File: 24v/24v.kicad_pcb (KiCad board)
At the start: 2 copper layers, 82.6 x 50.8 mm, 51 parts, among them J1 Conn_01x08_Female, J2 Conn_01x01, J3 Conn_02x08_Counter_Clockwise, J4 Conn_02x08_Counter_Clockwise, J5 Conn_01x01, J6 Conn_02x08_Counter_Clockwise, J7 Conn_02x08_Counter_Clockwise, Q1 FET_A_UP, Q2 FET_A_DOWN, Q3 FET_B_UP, Q4 FET_B_DOWN, U1 7400, U2 IRS2108, U3 TLP2955, U4 TLP2955, U5 IRS2108, U6 L7812

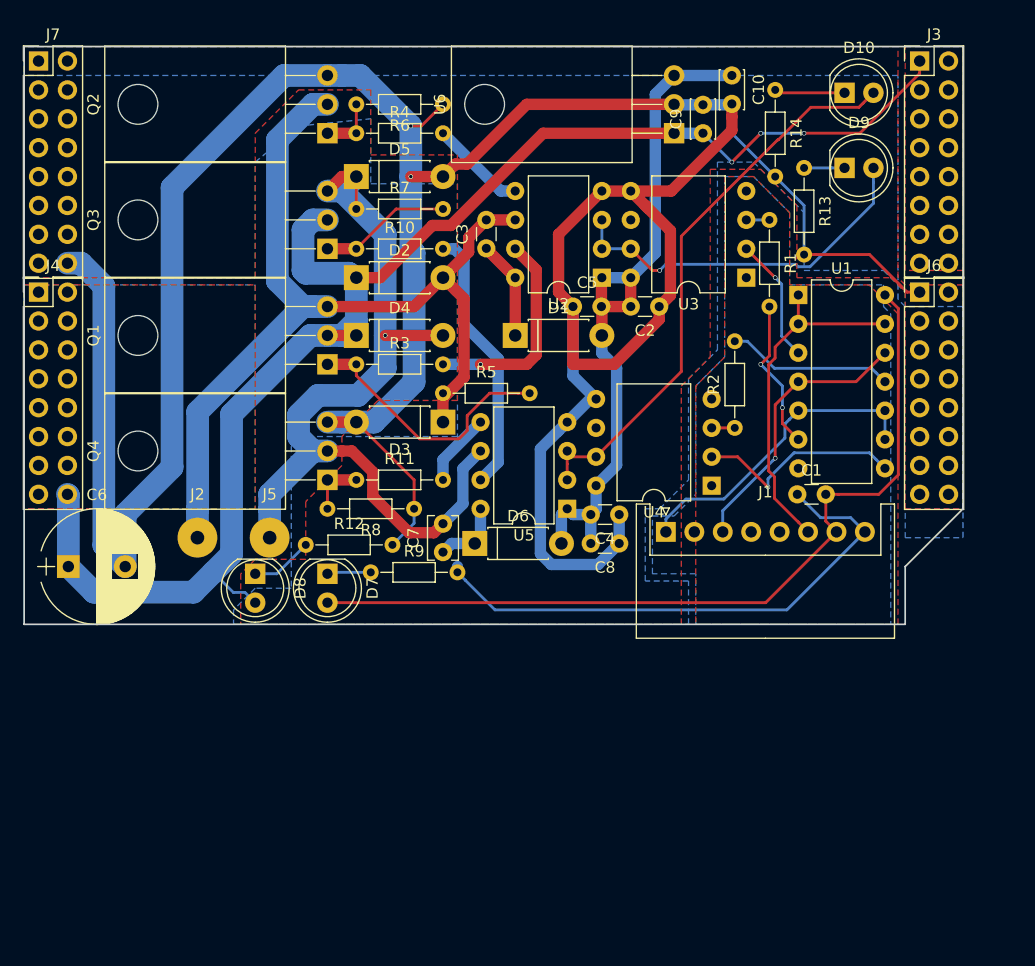
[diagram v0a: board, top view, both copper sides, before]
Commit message: design 24v ver
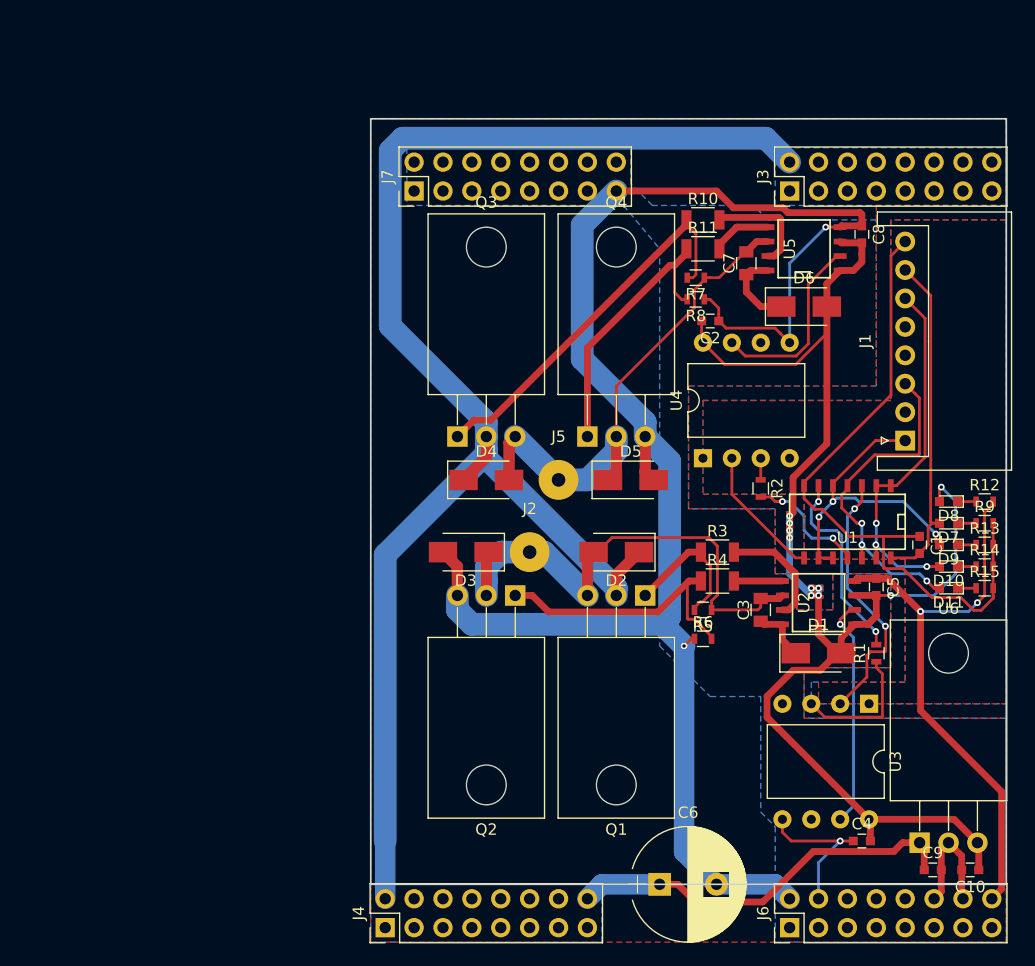
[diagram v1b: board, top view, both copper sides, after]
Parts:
- added D11: LED, LEDs:LED_0603, F.Cu at (144.8, 123.8)
- added R15: R, Resistors_SMD:R_0603, F.Cu at (148.0, 123.8)
- C1, C2, C4, C5, C8: footprint Capacitors_THT:C_Disc_D3.0mm_W1.6mm_P2.50mm -> Capacitors_SMD:C_0603
- C10: value relgoutC -> RegOutC; footprint Capacitors_THT:C_Disc_D3.4mm_W2.1mm_P2.50mm -> Capacitors_SMD:C_0603
- C3: footprint Capacitors_THT:C_Disc_D3.0mm_W1.6mm_P2.50mm -> Capacitors_SMD:C_0805
- C7: footprint Capacitors_THT:C_Disc_D3.8mm_W2.6mm_P2.50mm -> Capacitors_SMD:C_0805
- C9: value reglinC -> RegInC; footprint Capacitors_THT:C_Disc_D3.4mm_W2.1mm_P2.50mm -> Capacitors_SMD:C_0603
- D1, D2, D3, D4, D5, D6: footprint Diodes_THT:D_DO-41_SOD81_P7.62mm_Horizontal -> Diodes_SMD:D_SMA
- D10, D7, D8, D9: footprint LEDs:LED_D5.0mm -> LEDs:LED_0603
- R1, R12, R13, R14, R2, R5, R6, R7, R8: footprint Resistors_THT:R_Axial_DIN0204_L3.6mm_D1.6mm_P7.62mm_Horizontal -> Resistors_SMD:R_0603
- R10, R11, R3, R4: footprint Resistors_THT:R_Axial_DIN0204_L3.6mm_D1.6mm_P7.62mm_Horizontal -> Resistors_SMD:R_1206
- R9: value R -> LEDR; footprint Resistors_THT:R_Axial_DIN0204_L3.6mm_D1.6mm_P7.62mm_Horizontal -> Resistors_SMD:R_0603
- U1: footprint Housings_DIP:DIP-14_W7.62mm -> SMD_Packages:SOIC-14_N
- U2, U5: value IRS2108 -> IRS2302; footprint Housings_DIP:DIP-8_W7.62mm -> SMD_Packages:SOIC-8-N
- U6: value L7812 -> LM7812_TO220
- moved C10 72.9 mm to (146.7, 148.6), turned to 180 degrees
- moved C9 67.8 mm to (143.4, 148.6), turned to 0 degrees
- moved U6 66.0 mm to (142.2, 146.2), turned to 0 degrees
- moved J4 63.7 mm to (95.2, 153.7), turned to 90 degrees
- moved D8 61.3 mm to (144.8, 116.2), turned to 180 degrees
- moved R12 59.8 mm to (148.0, 116.2)
- moved C6 59.0 mm to (119.4, 149.9)
- moved J6 57.0 mm to (130.8, 153.7), turned to 90 degrees
- moved D7 54.8 mm to (144.8, 118.1), turned to 180 degrees
- moved R9 54.1 mm to (148.0, 118.1)
- moved R6 52.3 mm to (123.2, 128.3), turned to 0 degrees
- moved R4 50.6 mm to (124.5, 123.2)
- moved R14 45.8 mm to (148.0, 121.9), turned to 0 degrees
- moved Q2 43.9 mm to (106.7, 124.5), turned to 180 degrees
- moved D10 42.6 mm to (144.8, 121.9), turned to 180 degrees
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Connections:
- D10 pad 2: OUTB -> INB
- D8 pad 2: +24V -> +12V
- D9 pad 2: OUTA -> INA
- R13 pad 2: GNDPWR -> GND
- R14 pad 2: GNDPWR -> GND
- U2 pad 3: OUTA -> +12V
- U5 pad 3: OUTB -> +12V
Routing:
- net GNDPWR: track 292.5 -> 226.8 mm, vias 2 -> 5
- net +12V: track 62.5 -> 126.1 mm, vias 0 -> 10
- net +5V: track 74.4 -> 29.7 mm
- net +24V: track 131.9 -> 171.2 mm, vias 3 -> 0
- net Net-(C3-Pad2): track 84.8 -> 46.2 mm
- net OUTB: track 49.9 -> 16.7 mm
- net Net-(C7-Pad2): track 77.2 -> 45.0 mm, vias 1 -> 0
- net Net-(Q3-Pad1): track 11.6 -> 33.9 mm
- net Net-(Q2-Pad1): track 5.08 -> 24.4 mm
- net Net-(Q4-Pad1): track 5.08 -> 24.1 mm
- net Net-(R10-Pad2): track 23.6 -> 9.56 mm
- net OUTA: track 32.9 -> 20.2 mm
- net Net-(U1-Pad3): track 11.7 -> 23.5 mm, vias 1 -> 2
- net GND: track 47.9 -> 58.8 mm
- net Net-(Q1-Pad1): track 23.5 -> 12.6 mm
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- added copper zone on B.Cu, net +12V
- added copper zone on F.Cu, net +12V
- removed copper zone on F.Cu, net +24V
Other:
- board size 82.6 x 50.8 mm -> 55.9 x 67.3 mm
- net class Default: via_dia 0.4 -> 0.6
- net class Power: via_dia 0.4 -> 0.6
- rule trace_min: 0.2 -> 0
- rule via_min_size: 0.4 -> 0.6
